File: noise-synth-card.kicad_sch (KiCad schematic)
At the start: 45 parts, among them J1 CVpitch, J2 FM in, J3 PWM in, J4 synth-power-header, J5 SawOut, J6 SquareOut, M1 imogen-wren-card, Q1 BC558, Q2 BC548, U1 HEF4093B, U2 TL074

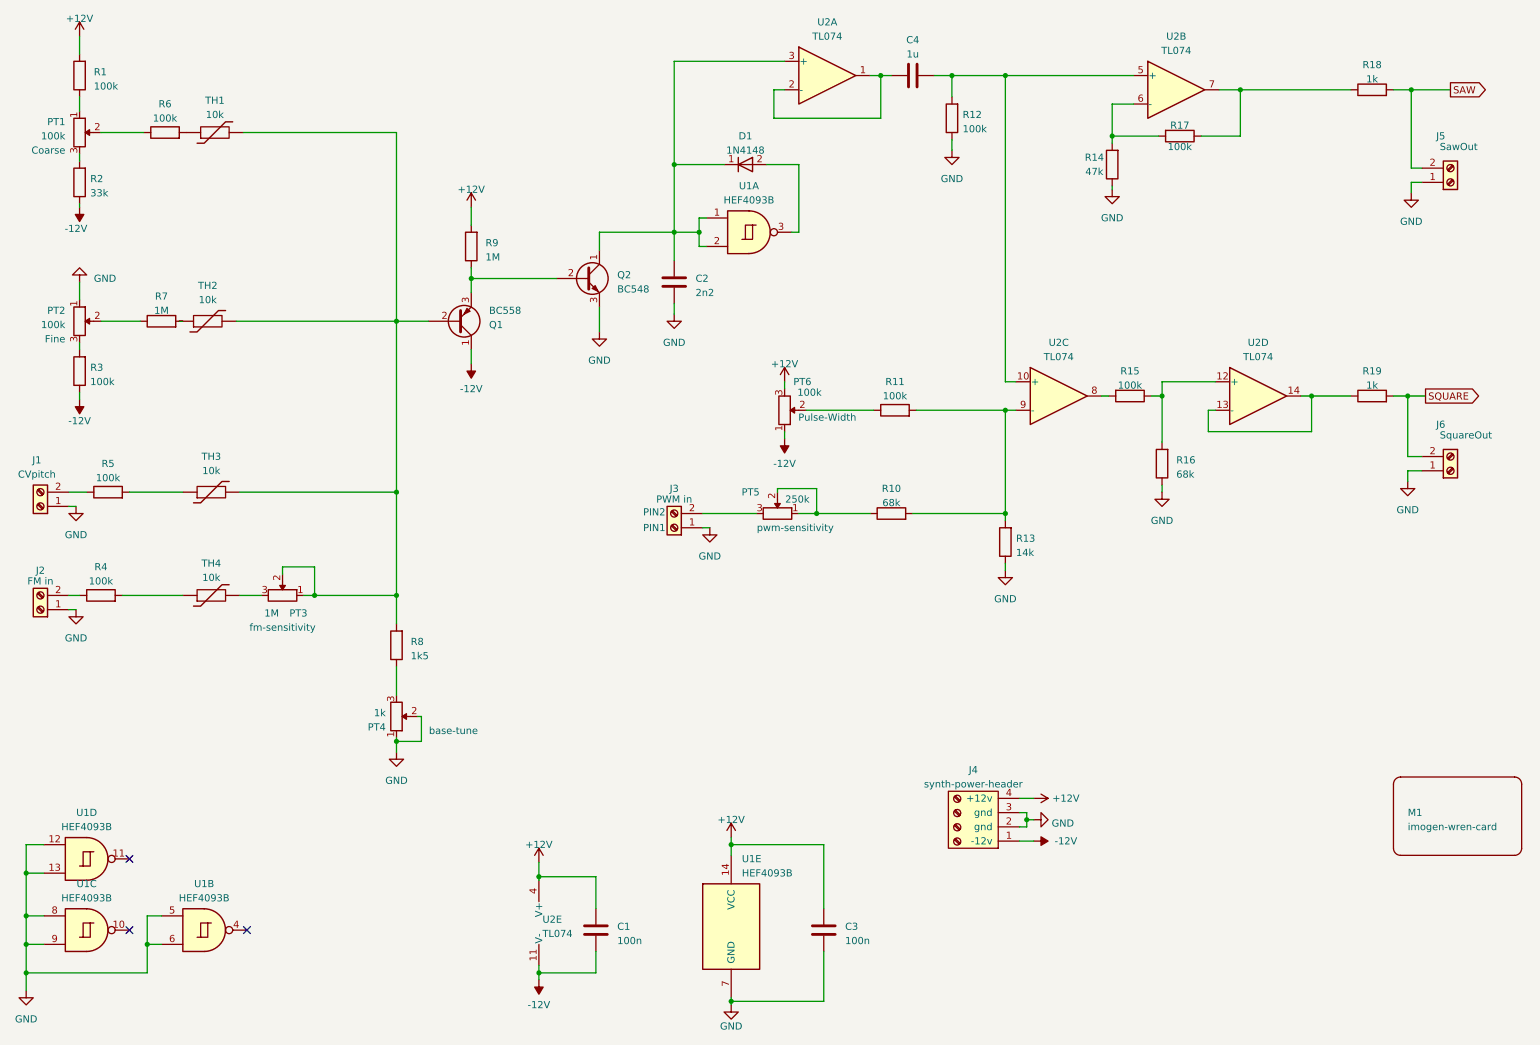
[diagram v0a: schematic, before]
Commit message: rtertert
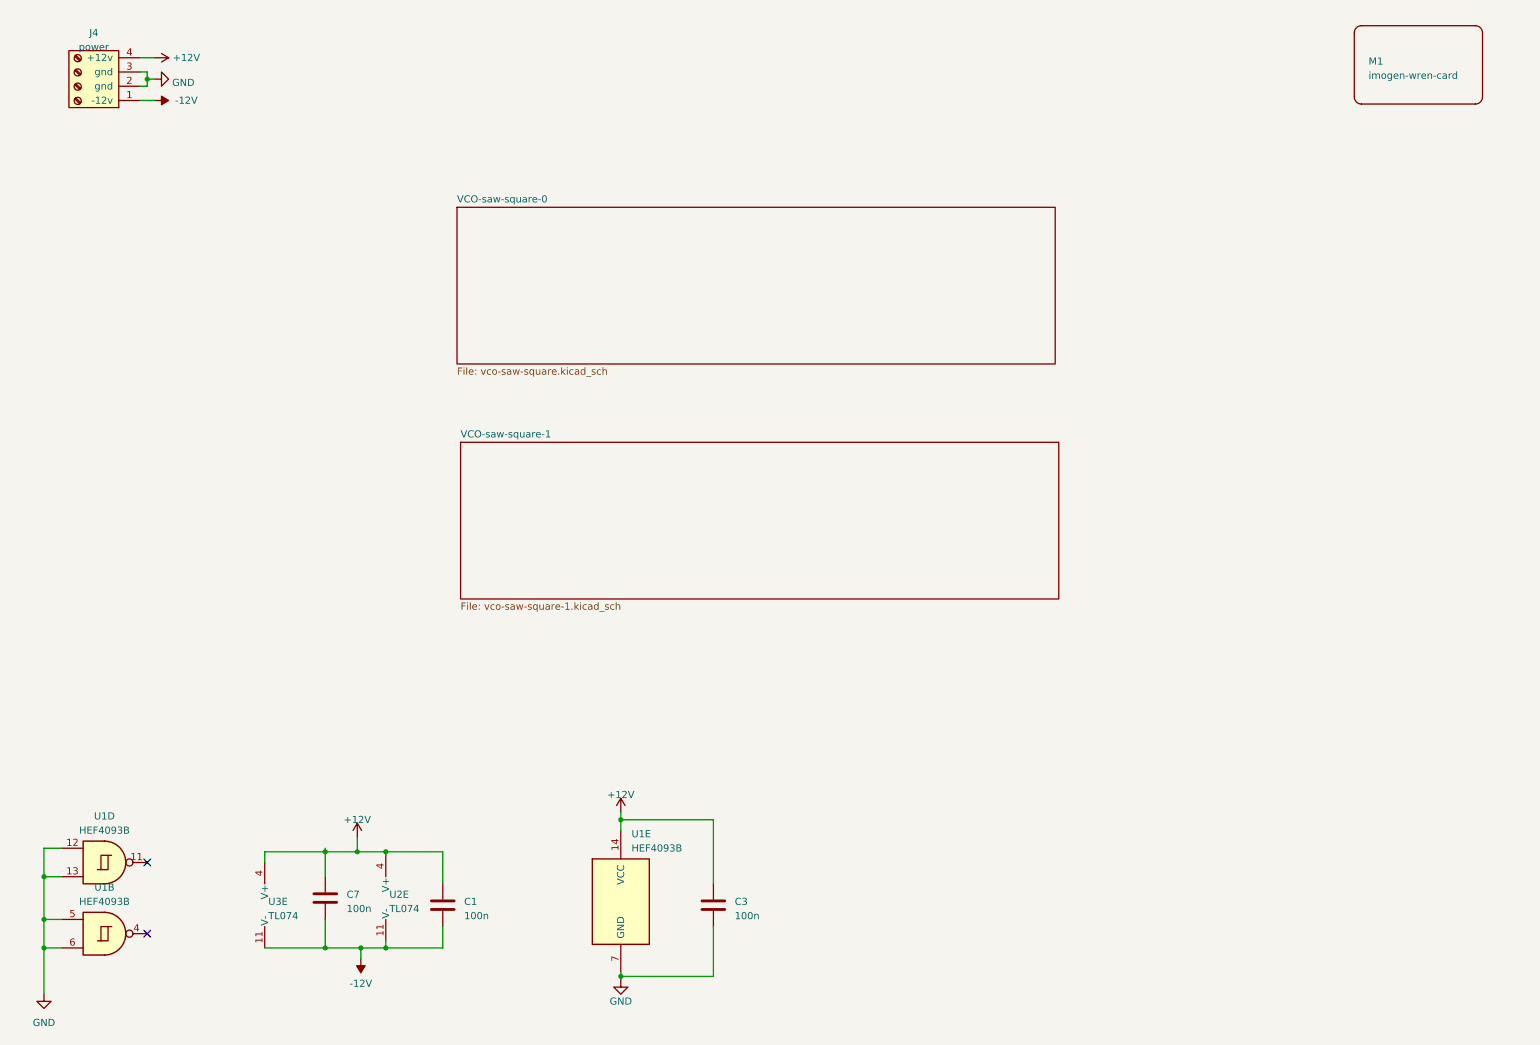
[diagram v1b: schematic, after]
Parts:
- removed C2: 2n2, 000_Capacitors_Immo:C_0805_2012_HandSolder_kawaii, symbol 000_Capacitor_Film_Immo:100n
- removed C4: 1u, Capacitor_SMD:C_0805_2012Metric_Pad1.18x1.45mm_HandSolder, symbol 000_Capacitor_Film_Immo:cap_film_0805
- removed D1: 1N4148, Diode_THT:D_DO-35_SOD27_P7.62mm_Horizontal, symbol 000_Diodes_Immo:1N4148
- removed J1: CVpitch, 000-screw-terminals-immo:TerminalBlock_Phoenix_MPT-0,5-2-2.54_1x02_P2.54mm_Horizontal, symbol 000-screw-terminals-immo:Screw_Terminal_01x02_small
- removed J2: FM in, 000-screw-terminals-immo:TerminalBlock_Phoenix_MPT-0,5-2-2.54_1x02_P2.54mm_Horizontal, symbol 000-screw-terminals-immo:Screw_Terminal_01x02_small
- removed J3: PWM in, 000-screw-terminals-immo:TerminalBlock_Phoenix_MPT-0,5-2-2.54_1x02_P2.54mm_Horizontal, symbol 000-screw-terminals-immo:Screw_Terminal_01x02_small
- removed J5: SawOut, 000-screw-terminals-immo:TerminalBlock_Phoenix_MPT-0,5-2-2.54_1x02_P2.54mm_Horizontal, symbol 000-screw-terminals-immo:Screw_Terminal_01x02_small
- removed J6: SquareOut, 000-screw-terminals-immo:TerminalBlock_Phoenix_MPT-0,5-2-2.54_1x02_P2.54mm_Horizontal, symbol 000-screw-terminals-immo:Screw_Terminal_01x02_small
- removed PT1, PT2, PT6: 100k, 000_Resistors_Immo:Potentiometer_Alpha-reversable, symbol 000_Resistors_Immo:Alpha Pot
- removed PT3: 1M, 000_Resistors_Immo:Potentiometer_Bourns-reversable-1, symbol 000_Resistors_Immo:50k_trimpot_MT
- removed PT4: 1k, 000_Resistors_Immo:Potentiometer_Bourns-reversable-1, symbol 000_Resistors_Immo:50k_trimpot_MT
- removed PT5: 250k, 000_Resistors_Immo:Potentiometer_Bourns-reversable-1, symbol 000_Resistors_Immo:50k_trimpot_MT
- removed Q1: BC558, Package_TO_SOT_THT:TO-92_Inline, symbol Transistor_BJT:BC558
- removed Q2: BC548, Package_TO_SOT_THT:TO-92_Inline, symbol Transistor_BJT:BC548
- removed R1, R11, R12, R15, R17, R3, R4, R5, R6: 100k, Resistor_SMD:R_0805_2012Metric_Pad1.20x1.40mm_HandSolder, symbol 000_Resistors_Immo:100k
- removed R10, R16: 68k, Resistor_SMD:R_0805_2012Metric_Pad1.20x1.40mm_HandSolder, symbol 000_Resistors_Immo:Resistor_0805
- removed R13: 14k, Resistor_SMD:R_0805_2012Metric_Pad1.20x1.40mm_HandSolder, symbol 000_Resistors_Immo:Resistor_0805
- removed R14: 47k, Resistor_SMD:R_0805_2012Metric_Pad1.20x1.40mm_HandSolder, symbol 000_Resistors_Immo:Resistor_0805
- removed R18, R19: 1k, Resistor_SMD:R_0805_2012Metric_Pad1.20x1.40mm_HandSolder, symbol 000_Resistors_Immo:Resistor_0805
- removed R2: 33k, Resistor_SMD:R_0805_2012Metric_Pad1.20x1.40mm_HandSolder, symbol 000_Resistors_Immo:Resistor_0805
- removed R7, R9: 1M, Resistor_SMD:R_0805_2012Metric_Pad1.20x1.40mm_HandSolder, symbol 000_Resistors_Immo:Resistor_0805
- removed R8: 1k5, Resistor_SMD:R_0805_2012Metric_Pad1.20x1.40mm_HandSolder, symbol 000_Resistors_Immo:Resistor_0805
- removed TH1, TH2, TH3, TH4: 10k, 000_Resistors_Immo:Resistor_0805_2012_handsolder, symbol 000-thermistor-immo:NTC-thermistor-10k-0805
- removed unit 1 of U1
- removed unit 3 of U1
- removed unit 4 of U2
- removed unit 1 of U2
- removed unit 3 of U2
- removed unit 2 of U2
- added C7: 100n, 000_Capacitors_Immo:C_0805_2012_HandSolder_kawaii, symbol 000_Capacitor_Film_Immo:100n
- added U3: TL074, Package_SO:SOIC-14_3.9x8.7mm_P1.27mm, symbol 000-op-amp-immo:TL074
- J4: value synth-power-header -> power
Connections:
- net +12V: now also C7.1, U3.4 (V+)
- net -12V: now also C7.2, U3.11 (V-)
- no-connect marks 3 -> 2
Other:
- added sheet VCO-saw-square-0 (vco-saw-square.kicad_sch)
- added sheet VCO-saw-square-1 (vco-saw-square-1.kicad_sch)
- moved on the sheet: C1, C3, J4, M1, U1B, U1D, U1E, U2E

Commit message: dsvgfsdgds
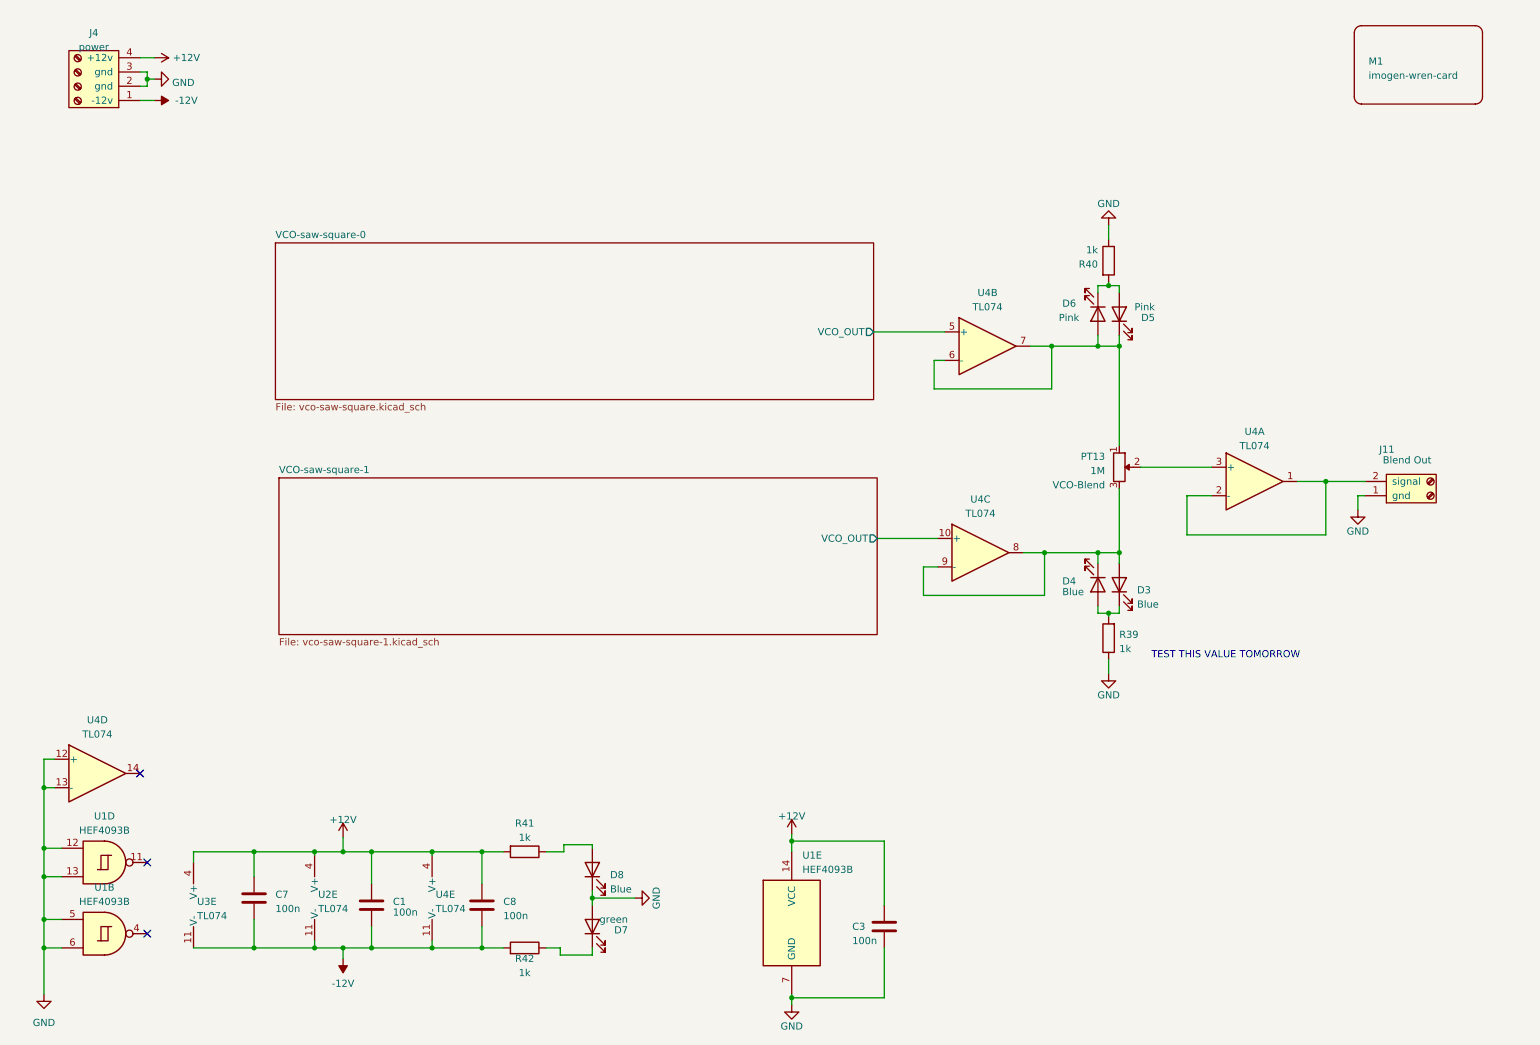
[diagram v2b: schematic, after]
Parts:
- added C8: 100n, 000_Capacitors_Immo:C_0805_2012_HandSolder_kawaii, symbol 000_Capacitor_Film_Immo:100n
- added D3, D4, D8: Blue, Diode_SMD:D_0805_2012Metric_Pad1.15x1.40mm_HandSolder, symbol 000_Diodes_Immo:LED_0805_Blue
- added D5, D6: Pink, Diode_SMD:D_0805_2012Metric_Pad1.15x1.40mm_HandSolder, symbol 000_Diodes_Immo:LED_0805_Blue
- added D7: green, Diode_SMD:D_0805_2012Metric_Pad1.15x1.40mm_HandSolder, symbol 000_Diodes_Immo:LED_0805_Blue
- added J11: Blend Out, 000-screw-terminals-immo:synth-signal-MPT-0,5-2-2.54_1x02_P2.54mm_Horizontal, symbol 000-screw-terminals-immo:synth-signal-header
- added PT13: 1M, 000_Resistors_Immo:Potentiometer_Alpha-reversable, symbol 000_Resistors_Immo:Alpha Pot
- added R39, R40, R41, R42: 1k, Resistor_SMD:R_0805_2012Metric_Pad1.20x1.40mm_HandSolder, symbol 000_Resistors_Immo:1k
- added U4: TL074, Package_SO:SOIC-14_3.9x8.7mm_P1.27mm, symbol 000-op-amp-immo:TL074
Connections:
- net +12V: now also C8.1, R41.2, U4.4 (V+)
- net -12V: now also C8.2, R42.2, U4.11 (V-)
- net GND: now also D7.2 (A), D8.1 (K), J11.1 (gnd), R39.1, R40.1, U4.12 (+), U4.13 (-)
- new net: D3.1 (K), D4.2 (A), R39.2
- new net: J11.2 (signal), U4.1, U4.2 (-)
- new net: D7.1 (K), R42.1
- new net: D5.1 (K), D6.2 (A), PT13.1, U4.6 (-), U4.7
- new net: D5.2 (A), D6.1 (K), R40.2
- new net: D3.2 (A), D4.1 (K), PT13.3, U4.8, U4.9 (-)
- new net: PT13.2, U4.3 (+)
- new net: D8.2 (A), R41.1
- new net VCO-saw-square-0/VCO_OUT: U4.5 (+)
- new net VCO-saw-square-1/VCO_OUT: U4.10 (+)
- no-connect marks 2 -> 3
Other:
- sheet VCO-saw-square-0 ports: added VCO_OUT; removed none
- sheet VCO-saw-square-1 ports: added VCO_OUT; removed none
- note added: "TEST THIS VALUE TOMORROW"
- moved on the sheet: C1, C3, C7, U1E, U2E, U3E
